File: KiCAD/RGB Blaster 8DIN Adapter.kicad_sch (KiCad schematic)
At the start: 6 parts, among them P1 Mini_DIN_9P_PCB, P2 8_pin_mini_DIN

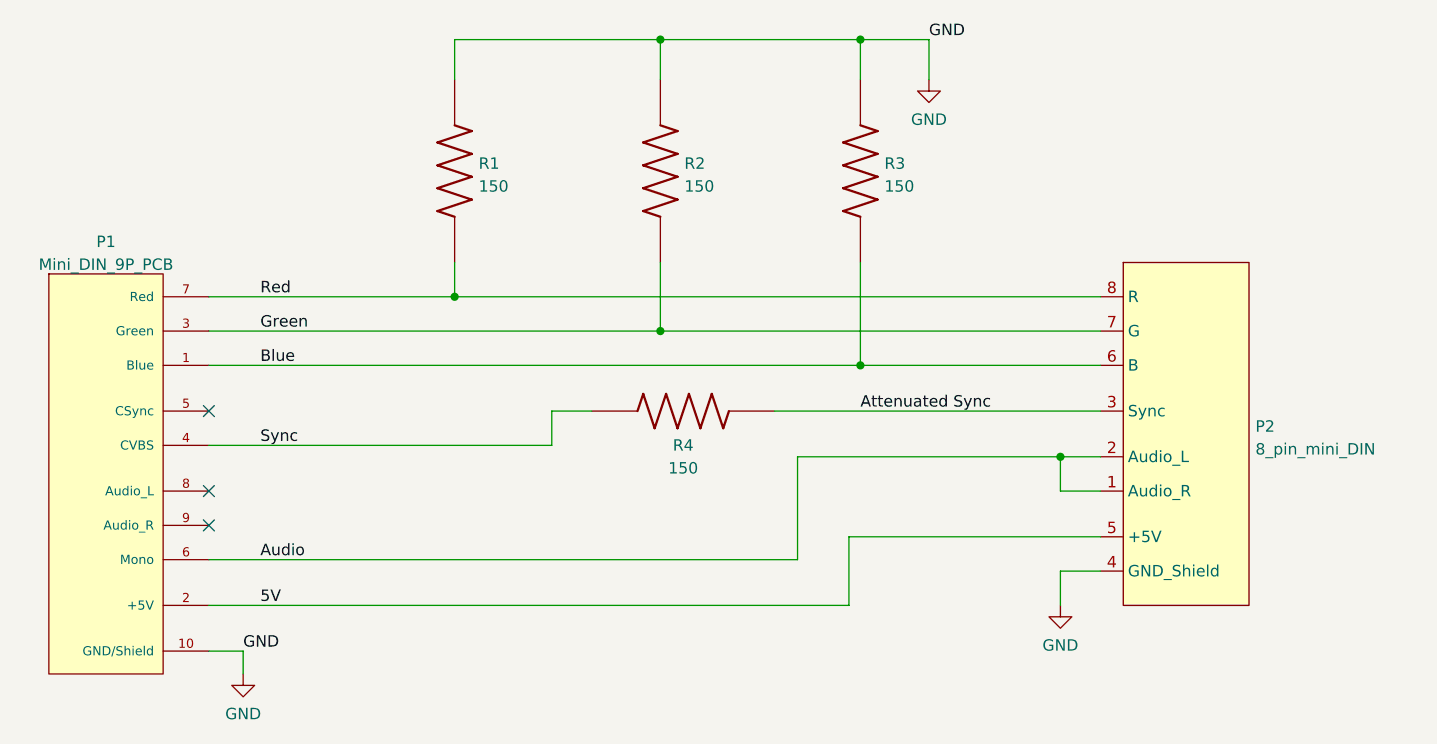
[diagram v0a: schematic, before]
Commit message: Changes on KiCAD project
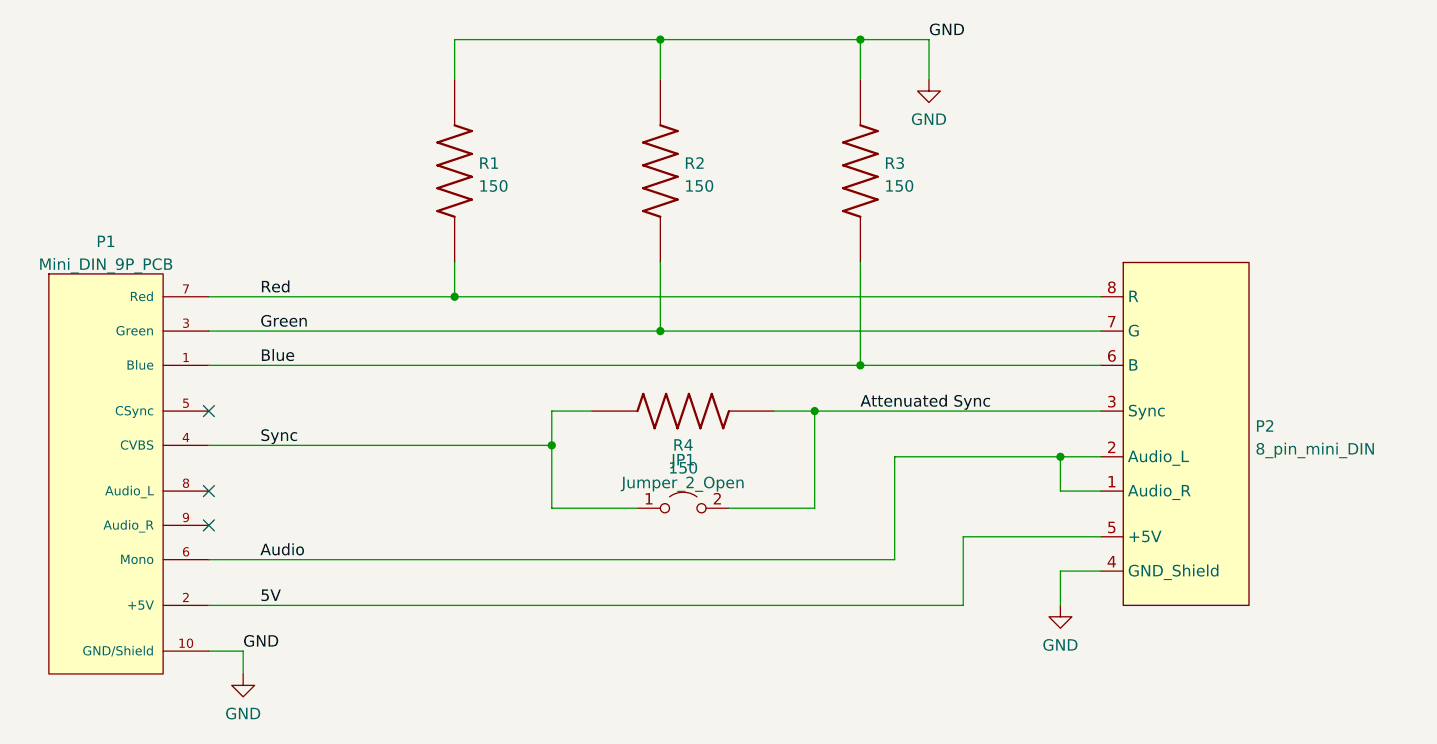
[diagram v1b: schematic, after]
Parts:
- added JP1: Jumper_2_Open, Jumper:SolderJumper-2_P1.3mm_Open_TrianglePad1.0x1.5mm, symbol Jumper:Jumper_2_Open
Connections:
- net Attenuated Sync: now also JP1.2 (B)
- net Sync: now also JP1.1 (A)
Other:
- company: (none) -> Jeff Chen
- title: (none) -> 8laster for RGB Blaster
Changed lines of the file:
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@@
 (kicad_sch (version 20211123) (generator eeschema)
   (paper "A4")
+  (title_block
+    (title "8laster for RGB Blaster")
+    (date "2023-01-29")
+    (rev "1")
+    (company "Jeff Chen")
+  )
   (junction (at 172.085 51.435) (diameter 0) (color 0 0 0 0)
   )
@@
   )
   (junction (at 149.86 83.82) (diameter 0) (color 0 0 0 0)
+  )
+  (junction (at 167.005 92.71) (diameter 0) (color 0 0 0 0)
+  )
+  (junction (at 137.795 96.52) (diameter 0) (color 0 0 0 0)
   )
   (junction (at 149.86 51.435) (diameter 0) (color 0 0 0 0)
@@
   (no_connect (at 99.695 101.6))
   (no_connect (at 99.695 92.71))
-  (wire (pts (xy 99.695 114.3) (xy 170.815 114.3))
+  (wire (pts (xy 99.695 114.3) (xy 183.515 114.3))
     (stroke (width 0) (type default) (color 0 0 0 0))
   )
@@
     (stroke (width 0) (type default) (color 0 0 0 0))
   )
+  (wire (pts (xy 157.48 103.505) (xy 167.005 103.505))
+    (stroke (width 0) (type default) (color 0 0 0 0))
+  )
   (wire (pts (xy 127 51.435) (xy 127 55.88))
     (stroke (width 0) (type default) (color 0 0 0 0))
@@
     (stroke (width 0) (type default) (color 0 0 0 0))
   )
-  (wire (pts (xy 162.56 92.71) (xy 198.755 92.71))
+  (wire (pts (xy 162.56 92.71) (xy 167.005 92.71))
     (stroke (width 0) (type default) (color 0 0 0 0))
   )
@@
     (stroke (width 0) (type default) (color 0 0 0 0))
   )
-  (wire (pts (xy 165.1 109.22) (xy 165.1 97.79))
+  (wire (pts (xy 175.895 109.22) (xy 175.895 97.79))
     (stroke (width 0) (type default) (color 0 0 0 0))
   )
@@
     (stroke (width 0) (type default) (color 0 0 0 0))
   )
+  (wire (pts (xy 167.005 92.71) (xy 198.755 92.71))
+    (stroke (width 0) (type default) (color 0 0 0 0))
+  )
   (wire (pts (xy 198.755 110.49) (xy 194.31 110.49))
     (stroke (width 0) (type default) (color 0 0 0 0))
   )
+  (wire (pts (xy 137.795 96.52) (xy 137.795 103.505))
+    (stroke (width 0) (type default) (color 0 0 0 0))
+  )
+  (wire (pts (xy 167.005 103.505) (xy 167.005 92.71))
+    (stroke (width 0) (type default) (color 0 0 0 0))
+  )
   (wire (pts (xy 99.695 80.01) (xy 127 80.01))
     (stroke (width 0) (type default) (color 0 0 0 0))
   )
-  (wire (pts (xy 99.695 109.22) (xy 165.1 109.22))
+  (wire (pts (xy 99.695 109.22) (xy 175.895 109.22))
     (stroke (width 0) (type default) (color 0 0 0 0))
   )
@@
     (stroke (width 0) (type default) (color 0 0 0 0))
   )
-  (wire (pts (xy 165.1 97.79) (xy 194.31 97.79))
+  (wire (pts (xy 175.895 97.79) (xy 194.31 97.79))
     (stroke (width 0) (type default) (color 0 0 0 0))
   )
@@
     (stroke (width 0) (type default) (color 0 0 0 0))
   )
-  (wire (pts (xy 170.815 106.68) (xy 198.755 106.68))
+  (wire (pts (xy 183.515 106.68) (xy 198.755 106.68))
     (stroke (width 0) (type default) (color 0 0 0 0))
   )
@@
     (stroke (width 0) (type default) (color 0 0 0 0))
   )
+  (wire (pts (xy 137.795 103.505) (xy 147.32 103.505))
+    (stroke (width 0) (type default) (color 0 0 0 0))
+  )
   (wire (pts (xy 172.085 51.435) (xy 172.085 55.88))
     (stroke (width 0) (type default) (color 0 0 0 0))
@@
     (stroke (width 0) (type default) (color 0 0 0 0))
   )
-  (wire (pts (xy 170.815 114.3) (xy 170.815 106.68))
+  (wire (pts (xy 183.515 114.3) (xy 183.515 106.68))
     (stroke (width 0) (type default) (color 0 0 0 0))
   )
@@
     (pin "2")
   )
+  (symbol (lib_id "Jumper:Jumper_2_Open") (at 152.4 103.505 0) (unit 1)
+    (in_bom yes) (on_board yes) (fields_autoplaced)
+    (property "Reference" "JP1" (id 0) (at 152.4 98.1542 0))
+    (property "Value" "Jumper_2_Open" (id 1) (at 152.4 100.6911 0))
+    (property "Footprint" "Jumper:SolderJumper-2_P1.3mm_Open_TrianglePad1.0x1.5mm" (id 2) (at 152.4 103.505 0)
+      (effects (font (size 1.27 1.27)) hide)
+    )
+    (property "Datasheet" "~" (id 3) (at 152.4 103.505 0)
+      (effects (font (size 1.27 1.27)) hide)
+    )
+    (pin "1")
+    (pin "2")
+  )
   (symbol (lib_id "resistor:Resistor_0603") (at 127 66.04 90) (unit 1)
     (in_bom yes) (on_board yes) (fields_autoplaced)
@@
       (reference "#PWR0103") (unit 1) (value "GND") (footprint "")
     )
+    (path "/a82bf7a0-f677-4cc2-9f55-cd220634e3a2"
+      (reference "JP1") (unit 1) (value "Jumper_2_Open") (footprint "Jumper:SolderJumper-2_P1.3mm_Open_TrianglePad1.0x1.5mm")
+    )
     (path "/87ccef06-d847-48b6-8f13-57f581e9bf7b"
